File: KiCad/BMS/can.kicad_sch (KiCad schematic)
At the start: 10 parts, among them J3 430450400, J4 Conn_01x03, U2 ISO1050DUB

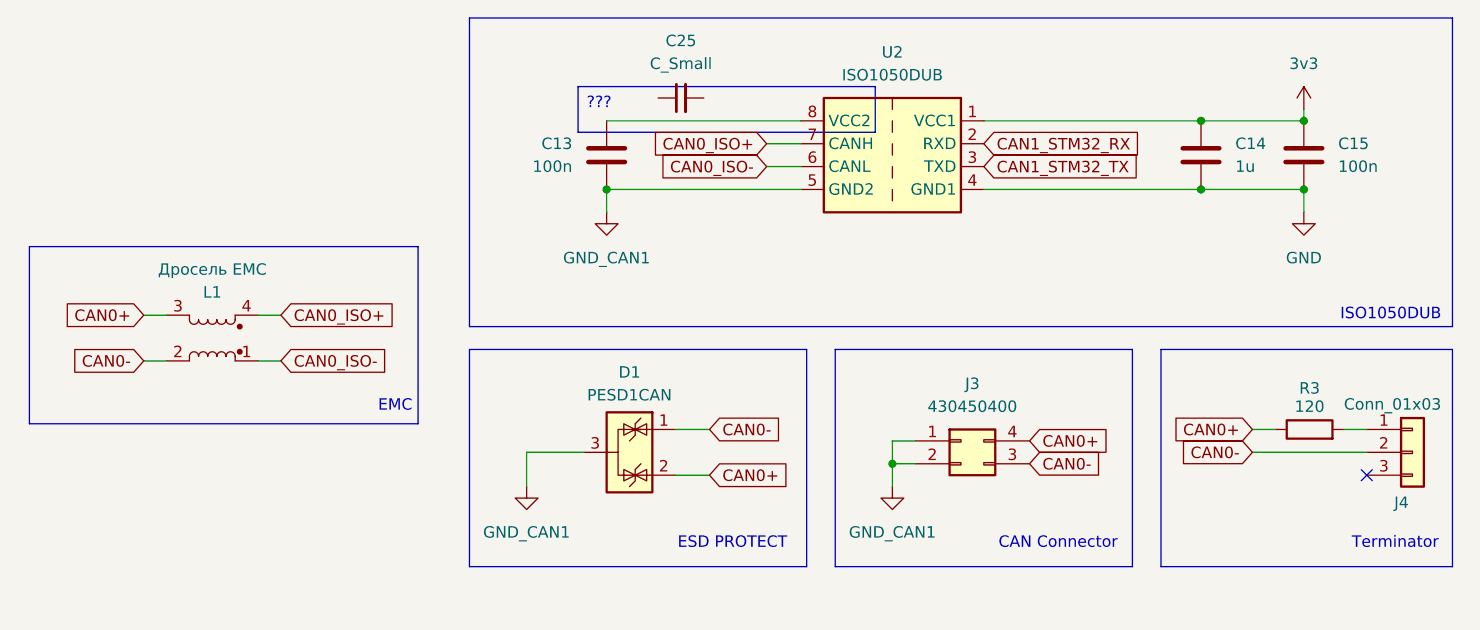
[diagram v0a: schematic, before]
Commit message: 23.03.2025
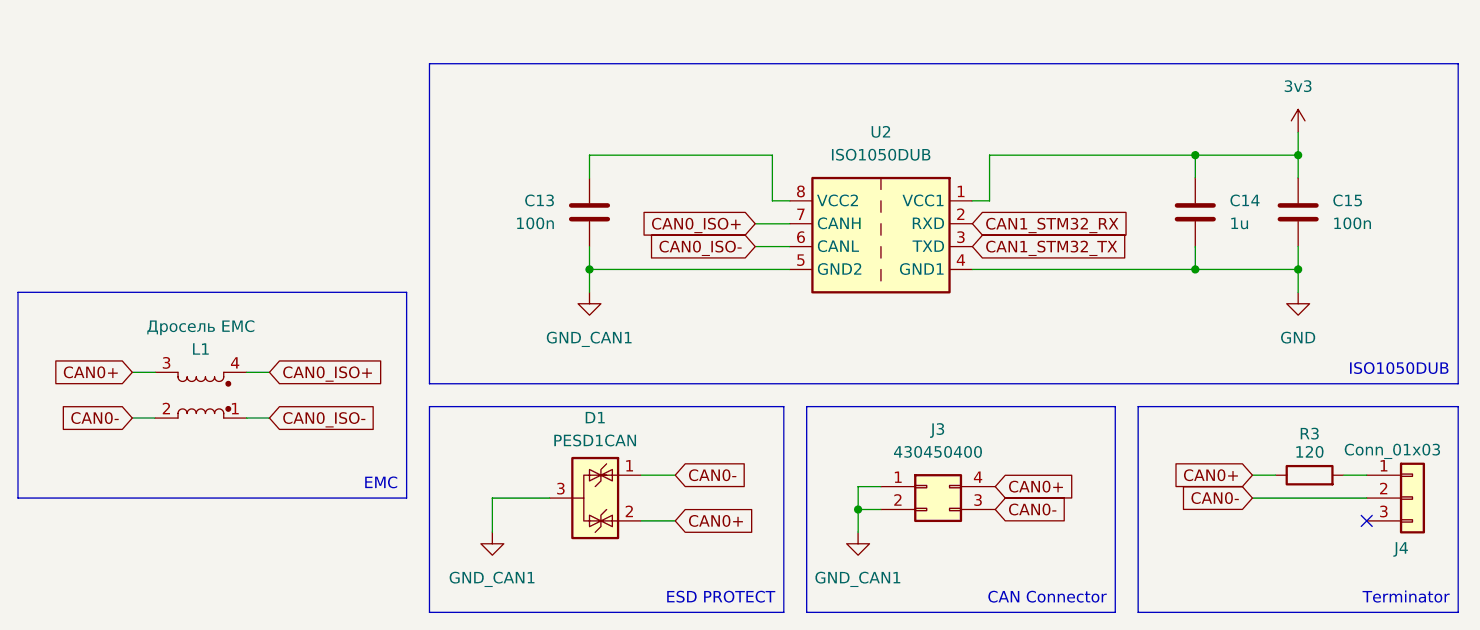
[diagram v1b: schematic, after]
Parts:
- removed C25: C_Small, symbol Device:C_Small
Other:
- note removed: "CAN Connector"
- note removed: "EMC"
- note removed: "ESD PROTECT"
- note removed: "ISO1050DUB"
- note removed: "Terminator"
- moved on the sheet: C13, C14, C15, D1, J3, J4, L1, R3, U2
